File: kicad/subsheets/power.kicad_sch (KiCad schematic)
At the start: 12 parts, among them U1 AP61300Z6, U2 AP61300Z6

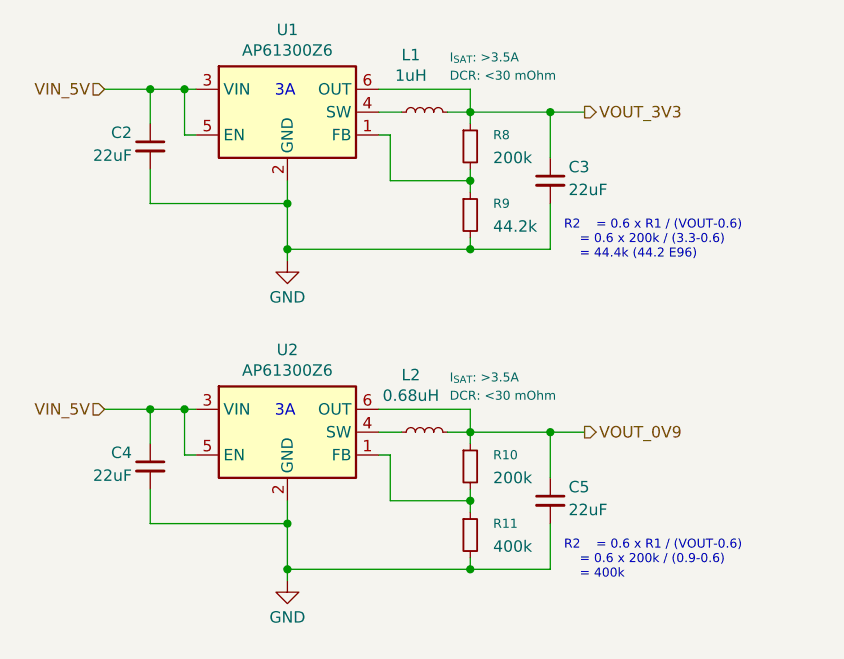
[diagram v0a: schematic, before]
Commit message: Start on PCB design
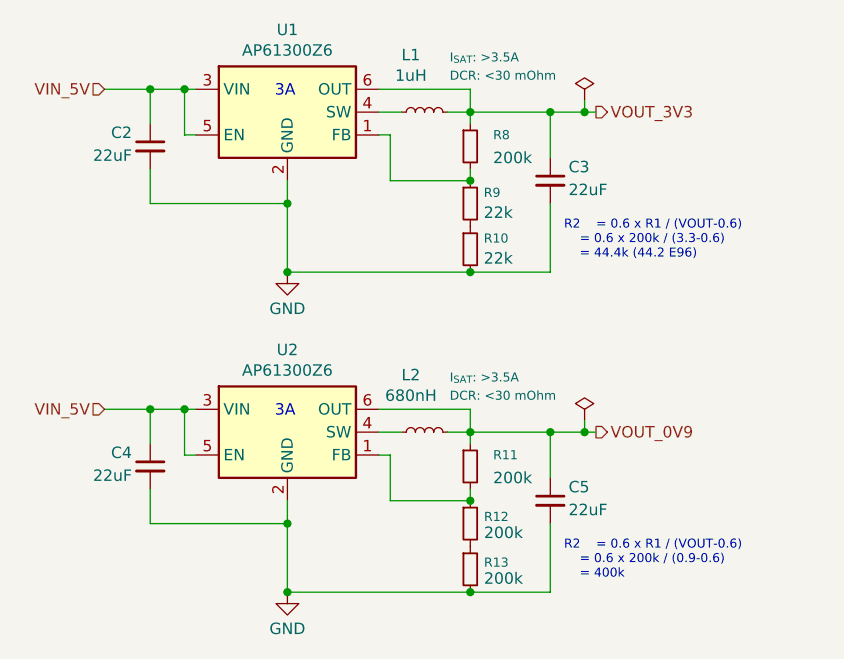
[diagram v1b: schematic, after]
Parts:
- removed R11: 400k, symbol Device:R_Small
- added R10: 22k, Resistor_SMD:R_0402_1005Metric, symbol Device:R_Small
- added R12, R13: 200k, Resistor_SMD:R_0402_1005Metric, symbol Device:R_Small
- C2, C3, C4, C5: footprint (none) -> Capacitor_SMD:C_1206_3216Metric; LCSC PART NAME (none) -> C12891
- L1: footprint (none) -> Inductor_SMD:L_0805_2012Metric; LCSC PART NAME (none) -> C1042
- L2: value 0.68uH -> 680nH; footprint (none) -> Inductor_SMD:L_0603_1608Metric; LCSC PART NAME (none) -> C55546
- R11: renamed from R10; footprint (none) -> Resistor_SMD:R_0402_1005Metric; LCSC PART NAME (none) -> C25764
- R8: footprint (none) -> Resistor_SMD:R_0402_1005Metric; LCSC PART NAME (none) -> C25764
- R9: value 44.2k -> 22k; footprint (none) -> Resistor_SMD:R_0402_1005Metric; LCSC PART NAME (none) -> C25768
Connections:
- net GND: now also R10.2, R13.2; no longer R9.2
- net at R11.2, U2.1 (FB): now also R12.1
- new net: R12.2, R13.1
- new net: R10.1, R9.2
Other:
- moved on the sheet: R9
